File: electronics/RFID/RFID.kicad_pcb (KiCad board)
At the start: 2 copper layers, 20 parts, among them J1 USB_C_Receptacle_PowerOnly_6P, J2 Conn_01x10_Pin, J4 Conn_01x16_Pin, U1 AP63200WU, U2 74LVC2G14

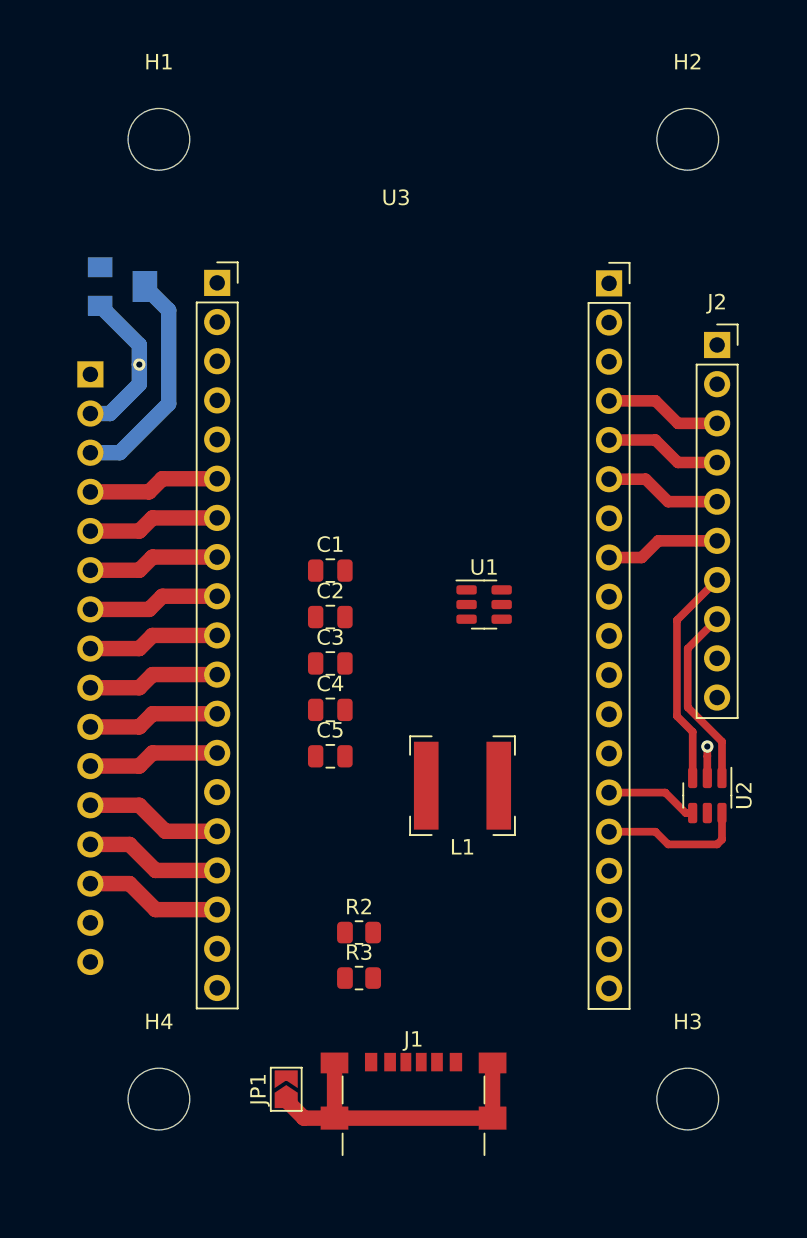
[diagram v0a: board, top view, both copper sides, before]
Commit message: pcb
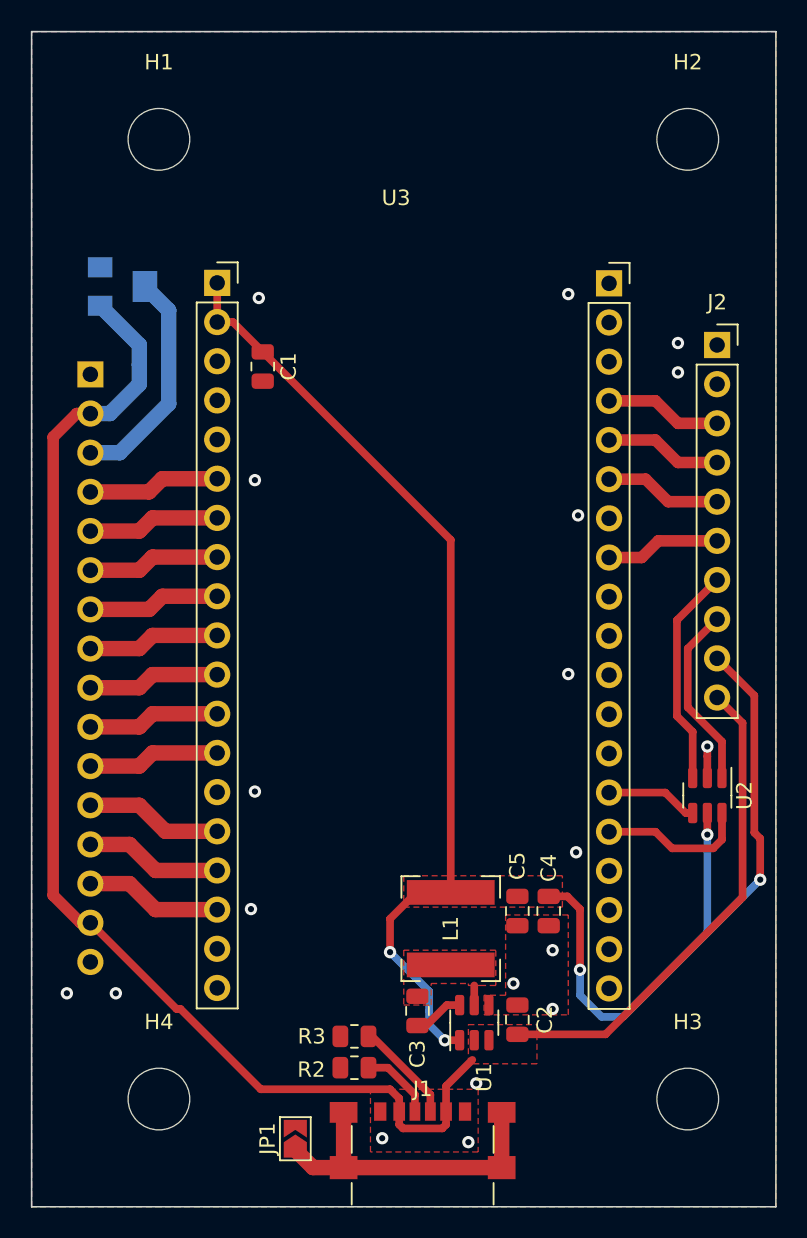
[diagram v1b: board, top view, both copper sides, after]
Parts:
- moved C2 28.8 mm to (124.2, 102.2), turned to 90 degrees
- moved U1 27.1 mm to (121.4, 102.4), turned to 90 degrees
- moved C3 23.2 mm to (117.7, 101.6), turned to -90 degrees
- moved C4 19.3 mm to (126.2, 95.1), turned to -90 degrees
- moved C5 15.7 mm to (124.2, 95.1), turned to -90 degrees
- moved C1 13.9 mm to (107.7, 59.8), turned to -90 degrees
- moved L1 9.30 mm to (119.9, 96.3), turned to 90 degrees
- moved R2 8.77 mm to (113.6, 105.3), turned to 180 degrees
- moved R3 3.79 mm to (113.6, 103.3), turned to 180 degrees
- moved J1 3.26 mm to (118.1, 111.2)
- moved JP1 3.26 mm to (109.8, 109.9)
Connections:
- C4 pad 1: /V3.3 -> +3.3V
- C5 pad 1: /V3.3 -> +3.3V
- L1 pad 2: /V3.3 -> +3.3V
- U1 pad 1: /V3.3 -> +3.3V
- U3 pad 2: unconnected-(U3-EN-Pad2) -> +3.3V
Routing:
- net +3.3V: track 0.00 -> 108.4 mm, vias 0 -> 5
- net +5V: track 10.1 -> 112.5 mm, vias 1 -> 0
- net Net-(J1-CC2): track 0.00 -> 6.67 mm
- net Net-(J1-CC1): track 0.00 -> 4.83 mm
- net Net-(U1-BST): track 0.00 -> 3.28 mm
- net Net-(U1-SW): track 0.00 -> 1.28 mm
- net GND: vias 1 -> 19
- added copper zone on F.Cu, net +3.3V
- added copper zone on F.Cu, net +5V
- added copper zone on B.Cu, net GND
- added copper zone on F.Cu, net GND
- added copper zone on F.Cu, net Net-(U1-SW)
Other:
- board outline added: 48.3 x 76.2 mm
